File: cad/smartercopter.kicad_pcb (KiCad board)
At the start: 2 copper layers, 37.7 x 16.8 mm, 74 parts, among them P1 CONN_5, P2 CONN_01X01, P3 CONN_01X01, P4 CONN_2, P5 CONN_01X01, P6 CONN_01X01, P7 CONN_01X01, Q1 SiA910EDJ, SW1 SW_PUSH_4, U1 CC2541, U2 MPU-9250, U3 TPS73001, U4 TPS73001, U5 DRV8837, X1 32Mhz

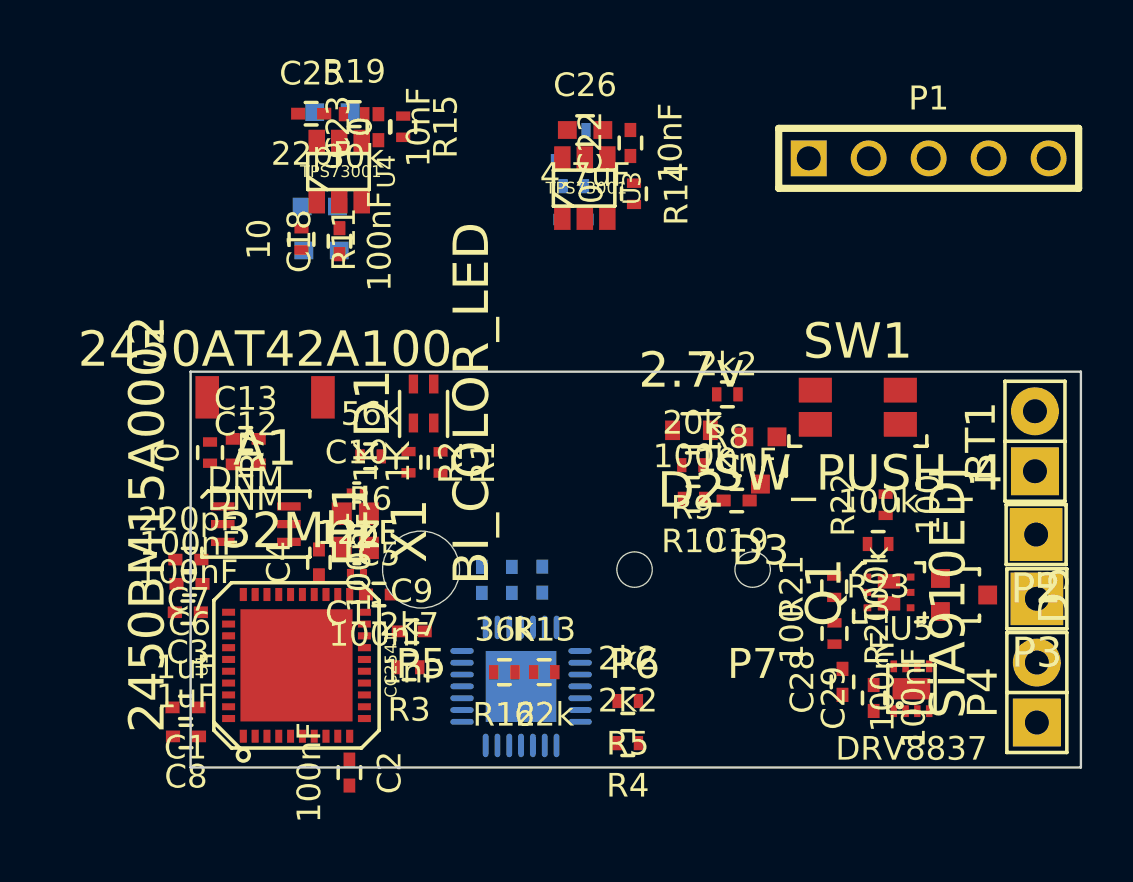
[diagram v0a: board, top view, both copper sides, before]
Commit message: everything on board
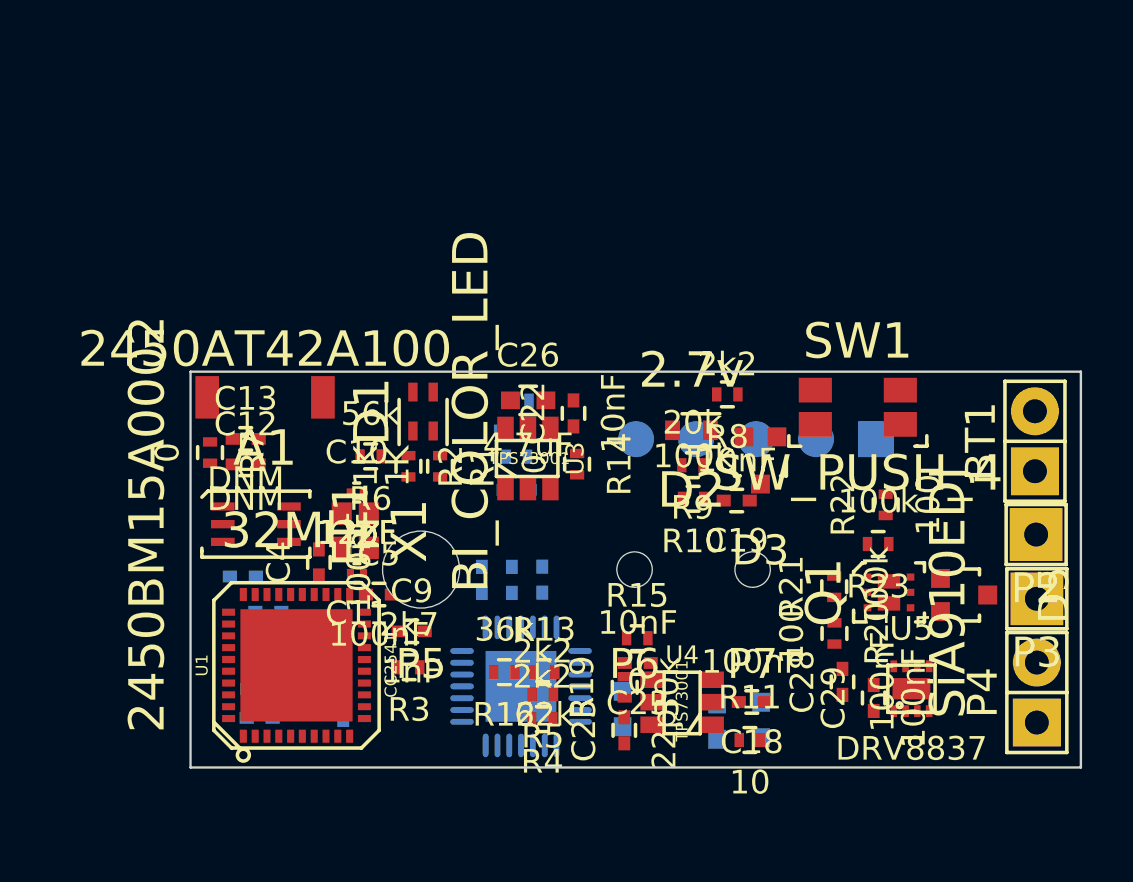
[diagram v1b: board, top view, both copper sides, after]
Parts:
- C1, C2, C3, C6, C7, C8, P1: moved to B.Cu
- moved C25 29.3 mm to (69.7, 119.7), turned to 90 degrees
- moved R11 28.5 mm to (75.0, 120.1), turned to 0 degrees
- moved C27 28.1 mm to (69.6, 118.8), turned to 90 degrees
- moved R18 27.9 mm to (70.8, 119.0), turned to 90 degrees
- moved C21 27.5 mm to (73.6, 119.3), turned to 90 degrees
- moved C17 27.2 mm to (75.5, 119.3), turned to 90 degrees
- moved R19 26.8 mm to (69.7, 117.9), turned to 90 degrees
- moved U4 26.8 mm to (72.1, 118.5), turned to 90 degrees
- moved C18 26.2 mm to (75.1, 118.5), turned to 180 degrees
- moved C23 25.2 mm to (70.2, 116.8), turned to 180 degrees
- moved R15 23.8 mm to (70.2, 115.8), turned to 0 degrees
- moved P1 14.0 mm to (75.3, 107.4), turned to 180 degrees
- moved R16 11.7 mm to (65.1, 108.1)
- moved U3 11.7 mm to (65.6, 108.2)
- moved C20 11.7 mm to (65.1, 109.5)
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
